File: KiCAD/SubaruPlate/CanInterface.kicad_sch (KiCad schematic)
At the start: 10 parts, among them J1 DF51A-4P-2DSA, U3 MCP2515-xSO, U4 MCP2562-E-SN, Y1 8MHz

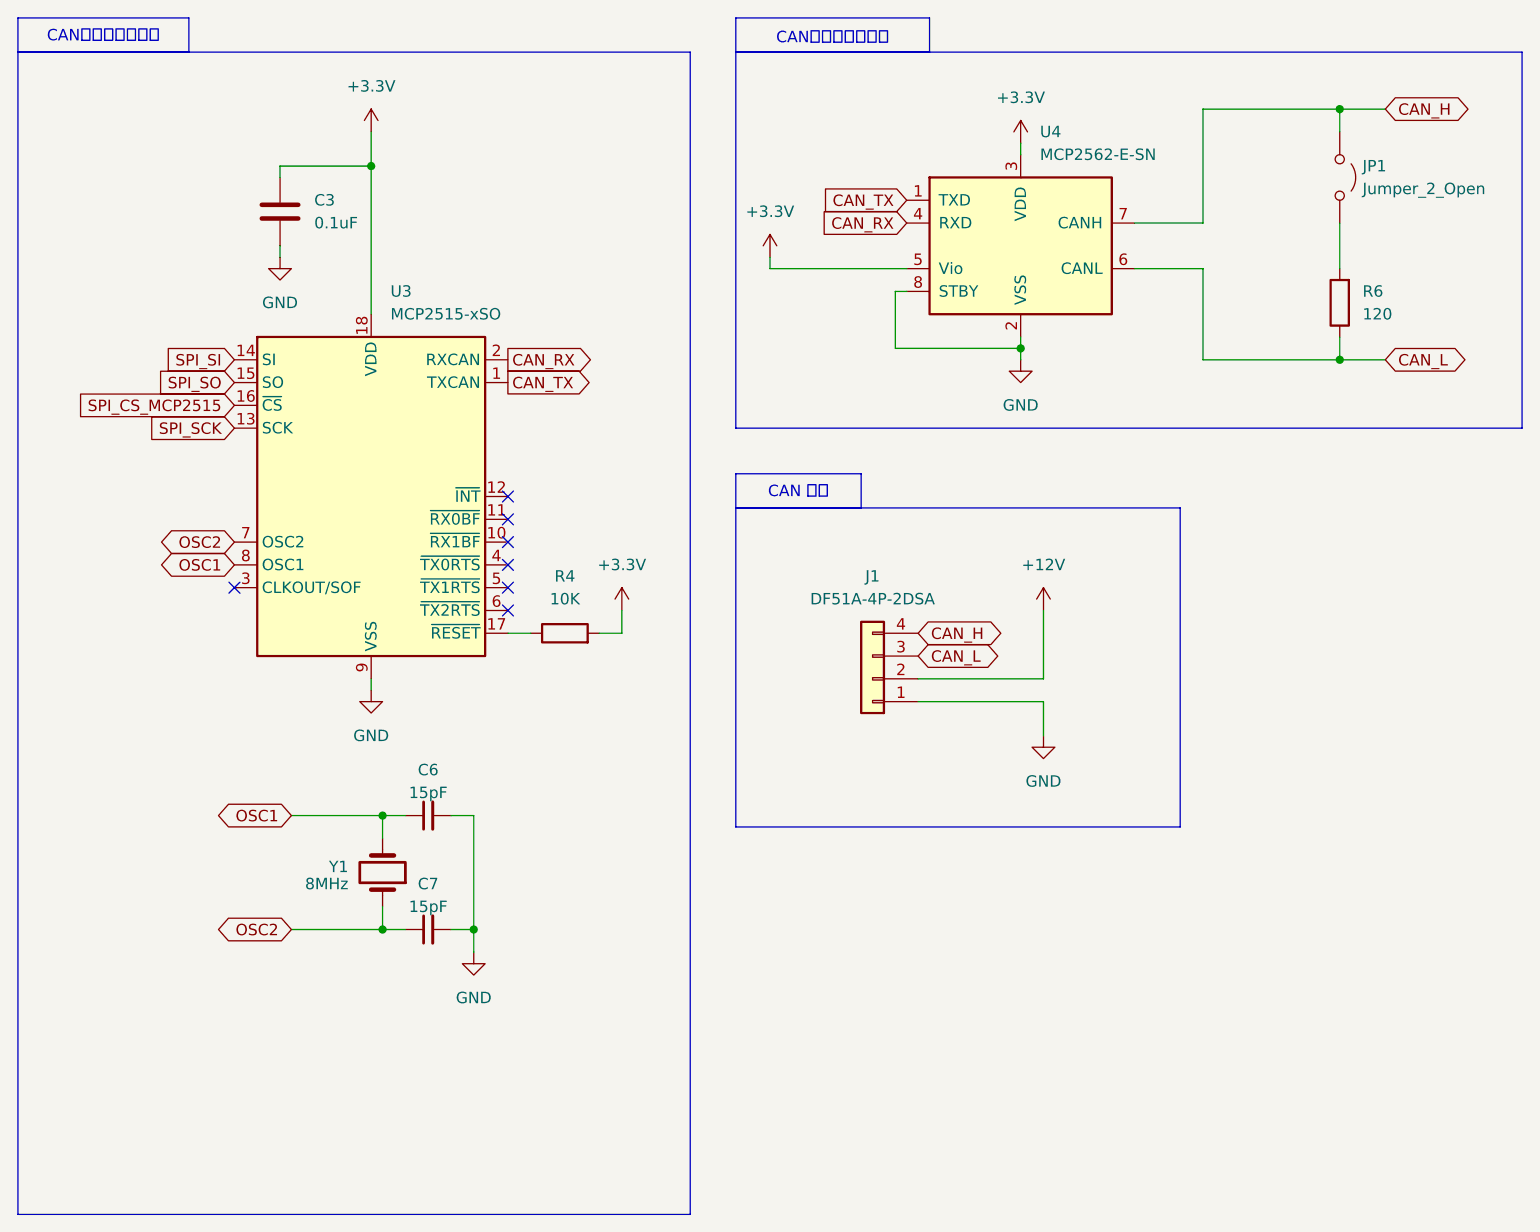
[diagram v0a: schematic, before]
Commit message: SubaruPlateを更新
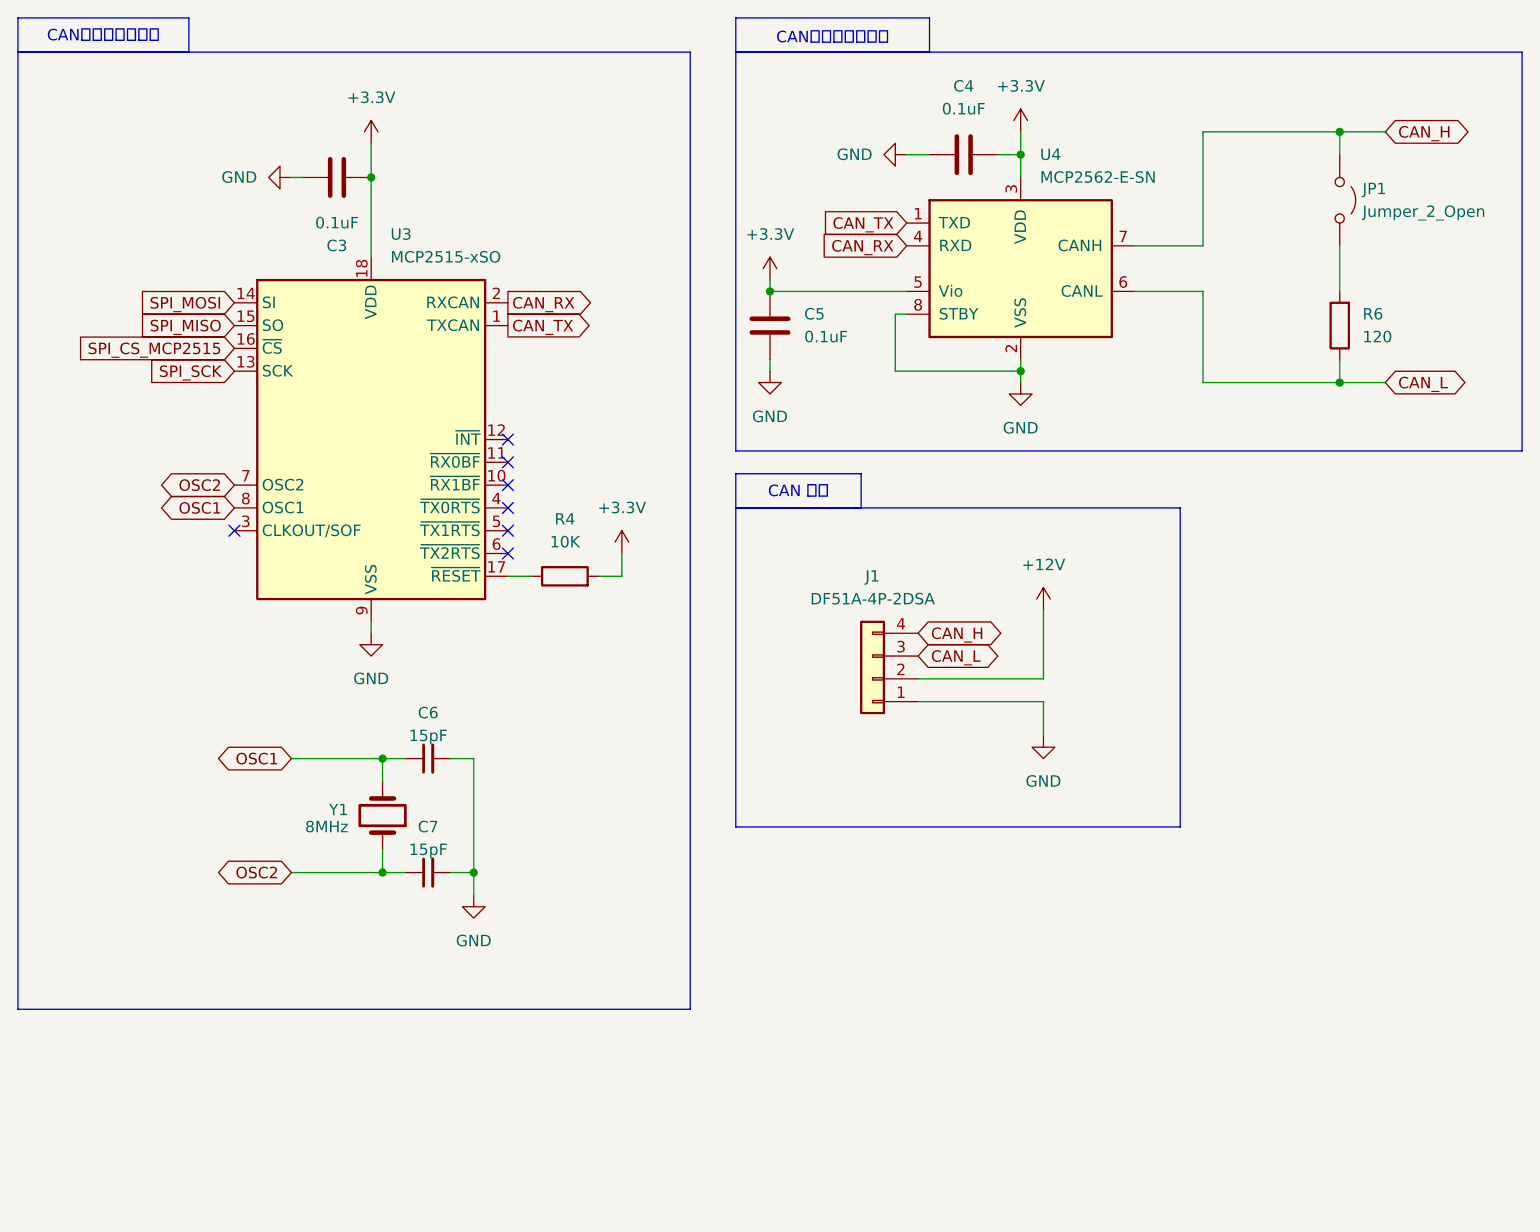
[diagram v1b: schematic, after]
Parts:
- added C4, C5: 0.1uF, Capacitor_SMD:C_0603_1608Metric_Pad1.08x0.95mm_HandSolder, symbol Device:C
- R4: footprint (none) -> Resistor_SMD:R_0603_1608Metric_Pad0.98x0.95mm_HandSolder
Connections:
- net +3.3V: now also C4.2, C5.2
- net GND: now also C4.1, C5.1
- net SPI_SI renamed SPI_MOSI
- net SPI_SO renamed SPI_MISO
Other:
- moved on the sheet: C3, C6, C7, JP1, R4, R6, U3, U4, Y1

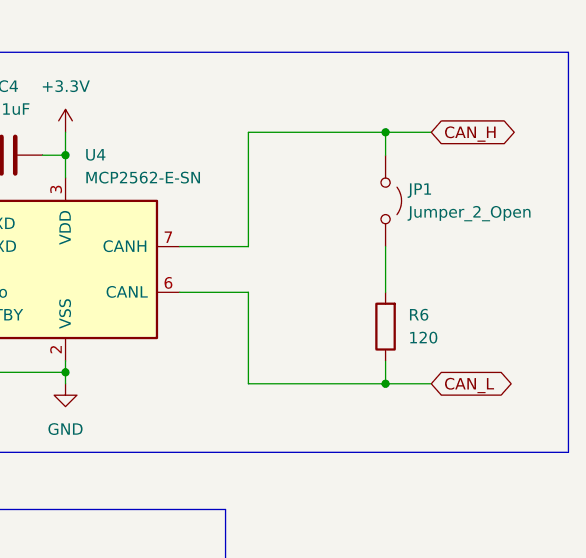
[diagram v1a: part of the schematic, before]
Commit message: 後は最終確認
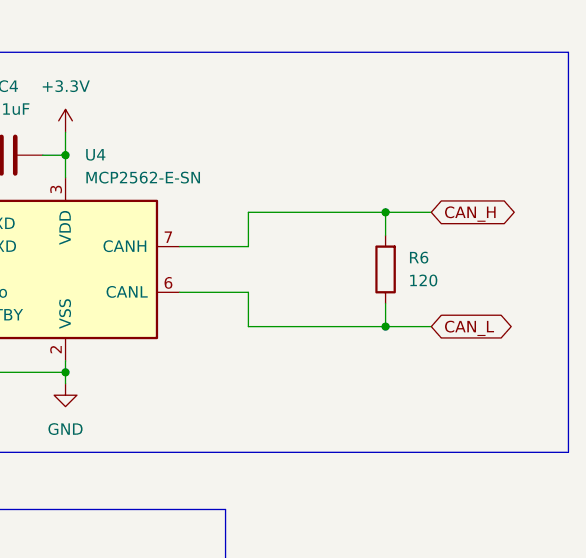
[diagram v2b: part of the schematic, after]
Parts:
- removed JP1: Jumper_2_Open, Jumper:SolderJumper-2_P1.3mm_Open_TrianglePad1.0x1.5mm, symbol Jumper:Jumper_2_Open
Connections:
- net CAN_H: now also R6.2
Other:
- moved on the sheet: R6
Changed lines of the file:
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@@
 	)
 	(junction
-		(at 177.8 60.96)
-		(diameter 0)
-		(color 0 0 0 0)
-	)
-	(junction
-		(at 177.8 33.02)
+		(at 177.8 54.61)
 		(diameter 0)
 		(color 0 0 0 0)
@@
 		(color 0 0 0 0)
 	)
+	(junction
+		(at 177.8 41.91)
+		(diameter 0)
+		(color 0 0 0 0)
+	)
 	(no_connect
 		(at 85.09 72.39)
@@
 	(wire
 		(pts
+			(xy 177.8 41.91) (xy 177.8 44.45)
+		)
+		(stroke
+			(width 0)
+			(type default)
+		)
+	)
+	(wire
+		(pts
 			(xy 69.85 38.1) (xy 69.85 46.99)
 		)
@@
 	(wire
 		(pts
-			(xy 177.8 45.72) (xy 177.8 50.8)
-		)
-		(stroke
-			(width 0)
-			(type default)
-		)
-	)
-	(wire
-		(pts
 			(xy 60.96 115.57) (xy 71.12 115.57)
 		)
@@
 	(wire
 		(pts
-			(xy 177.8 33.02) (xy 182.88 33.02)
+			(xy 177.8 41.91) (xy 182.88 41.91)
 		)
 		(stroke
@@
 	(wire
 		(pts
-			(xy 162.56 33.02) (xy 162.56 45.72)
+			(xy 162.56 41.91) (xy 162.56 45.72)
 		)
 		(stroke
@@
 	(wire
 		(pts
-			(xy 177.8 60.96) (xy 162.56 60.96)
+			(xy 177.8 54.61) (xy 162.56 54.61)
 		)
 		(stroke
@@
 	(wire
 		(pts
-			(xy 162.56 33.02) (xy 177.8 33.02)
+			(xy 162.56 41.91) (xy 177.8 41.91)
 		)
 		(stroke
@@
 	(wire
 		(pts
-			(xy 182.88 60.96) (xy 177.8 60.96)
+			(xy 182.88 54.61) (xy 177.8 54.61)
 		)
 		(stroke
@@
 	(wire
 		(pts
-			(xy 177.8 33.02) (xy 177.8 35.56)
-		)
-		(stroke
-			(width 0)
-			(type default)
-		)
-	)
-	(wire
-		(pts
 			(xy 97.79 82.55) (xy 97.79 80.01)
 		)
@@
 	(wire
 		(pts
-			(xy 162.56 60.96) (xy 162.56 50.8)
+			(xy 162.56 54.61) (xy 162.56 50.8)
 		)
 		(stroke
@@
 	(wire
 		(pts
-			(xy 177.8 58.42) (xy 177.8 60.96)
+			(xy 177.8 52.07) (xy 177.8 54.61)
 		)
 		(stroke
@@
 	(global_label "CAN_L"
 		(shape bidirectional)
-		(at 182.88 60.96 0)
+		(at 182.88 54.61 0)
 		(fields_autoplaced yes)
 		(effects
@@
 		)
 		(property "Intersheetrefs" "${INTERSHEET_REFS}"
-			(at 192.6613 60.96 0)
+			(at 192.6613 54.61 0)
 			(effects
 				(font
@@
 	(global_label "CAN_H"
 		(shape bidirectional)
-		(at 182.88 33.02 0)
+		(at 182.88 41.91 0)
 		(fields_autoplaced yes)
 		(effects
@@
 		)
 		(property "Intersheetrefs" "${INTERSHEET_REFS}"
-			(at 192.9637 33.02 0)
+			(at 192.9637 41.91 0)
 			(effects
 				(font
@@
 	(symbol
 		(lib_id "Device:R")
-		(at 177.8 54.61 180)
+		(at 177.8 48.26 180)
 		(unit 1)
 		(exclude_from_sim no)
@@
 		(fields_autoplaced yes)
 		(property "Reference" "R6"
-			(at 180.34 53.3399 0)
+			(at 180.34 46.9899 0)
 			(effects
 				(font
@@
 		)
 		(property "Value" "120"
-			(at 180.34 55.8799 0)
+			(at 180.34 49.5299 0)
 			(effects
 				(font
@@
 		)
 		(property "Footprint" "Resistor_SMD:R_0603_1608Metric_Pad0.98x0.95mm_HandSolder"
-			(at 179.578 54.61 90)
+			(at 179.578 48.26 90)
 			(effects
 				(font
@@
 		)
 		(property "Datasheet" "~"
-			(at 177.8 54.61 0)
+			(at 177.8 48.26 0)
 			(effects
 				(font
@@
 		)
 		(property "Description" "Resistor"
-			(at 177.8 54.61 0)
+			(at 177.8 48.26 0)
 			(effects
 				(font
@@
 					(unit 1)
 				)
-			)
-		)
-	)
-	(symbol
-		(lib_id "Jumper:Jumper_2_Open")
-		(at 177.8 40.64 270)
-		(unit 1)
-		(exclude_from_sim no)
-		(in_bom yes)
-		(on_board yes)
-		(dnp no)
-		(fields_autoplaced yes)
-		(property "Reference" "JP1"
-			(at 180.34 39.3699 90)
-			(effects
-				(font
-					(size 1.27 1.27)
-				)
-				(justify left)
-			)
-		)
-		(property "Value" "Jumper_2_Open"
-			(at 180.34 41.9099 90)
-			(effects
-				(font
-					(size 1.27 1.27)
-				)
-				(justify left)
-			)
-		)
-		(property "Footprint" "Jumper:SolderJumper-2_P1.3mm_Open_TrianglePad1.0x1.5mm"
-			(at 177.8 40.64 0)
-			(effects
-				(font
-					(size 1.27 1.27)
-				)
-				(hide yes)
-			)
-		)
-		(property "Datasheet" "~"
-			(at 177.8 40.64 0)
-			(effects
-				(font
-					(size 1.27 1.27)
-				)
-				(hide yes)
-			)
-		)
-		(property "Description" "Jumper, 2-pole, open"
-			(at 177.8 40.64 0)
-			(effects
-				(font
-					(size 1.27 1.27)
-				)
-				(hide yes)
-			)
-		)
-		(pin "2"
-		)
-		(pin "1"
-		)
-		(instances
-			(project ""
-				(path "/6c4aa1f5-c08b-4349-85f8-88bb399e711f/44ad5b2d-22cb-4ed2-bb54-706dcaaae99f"
-					(reference "JP1")
-					(unit 1)
-				)
